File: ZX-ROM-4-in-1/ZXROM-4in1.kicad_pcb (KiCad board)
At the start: 2 copper layers, 27.9 x 35.6 mm, 9 parts, among them IC5 27C512, J1 Conn_01x14, J2 Conn_01x14, SW1 SW_DIP_x02

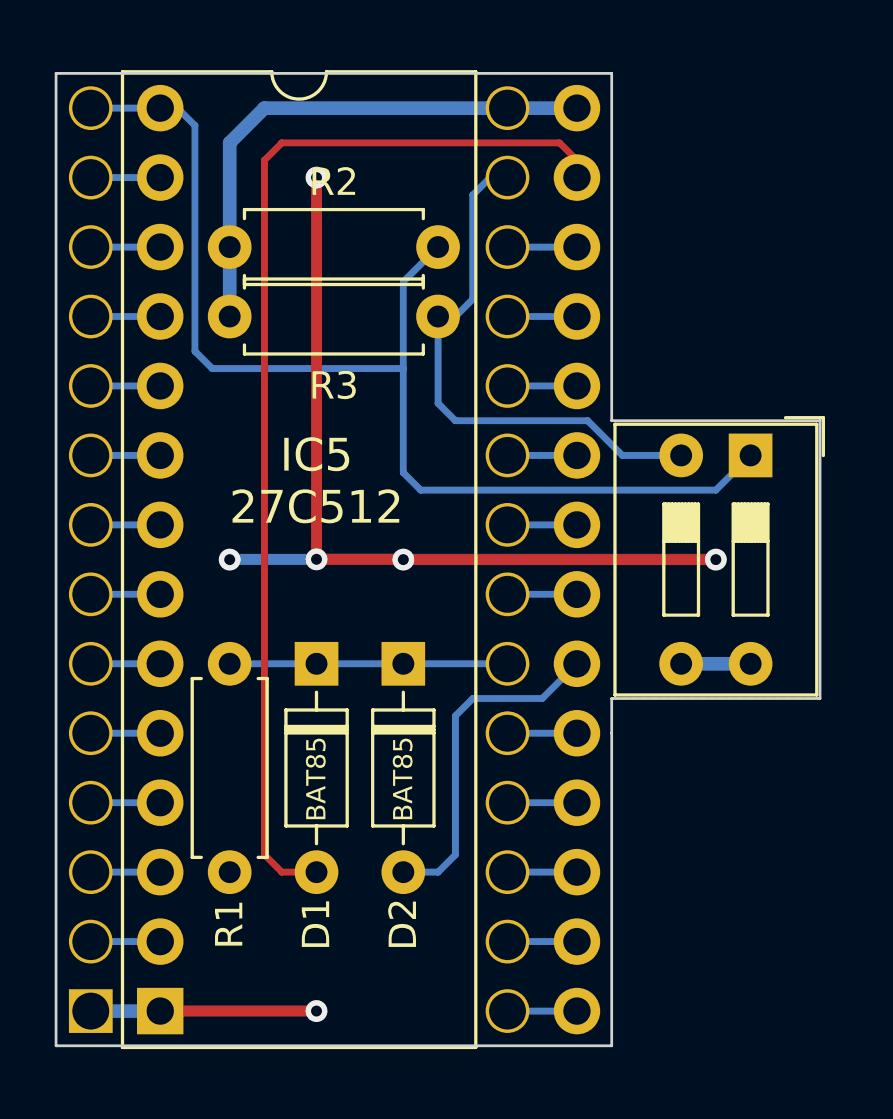
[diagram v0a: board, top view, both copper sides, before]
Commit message: New images, and adapter update
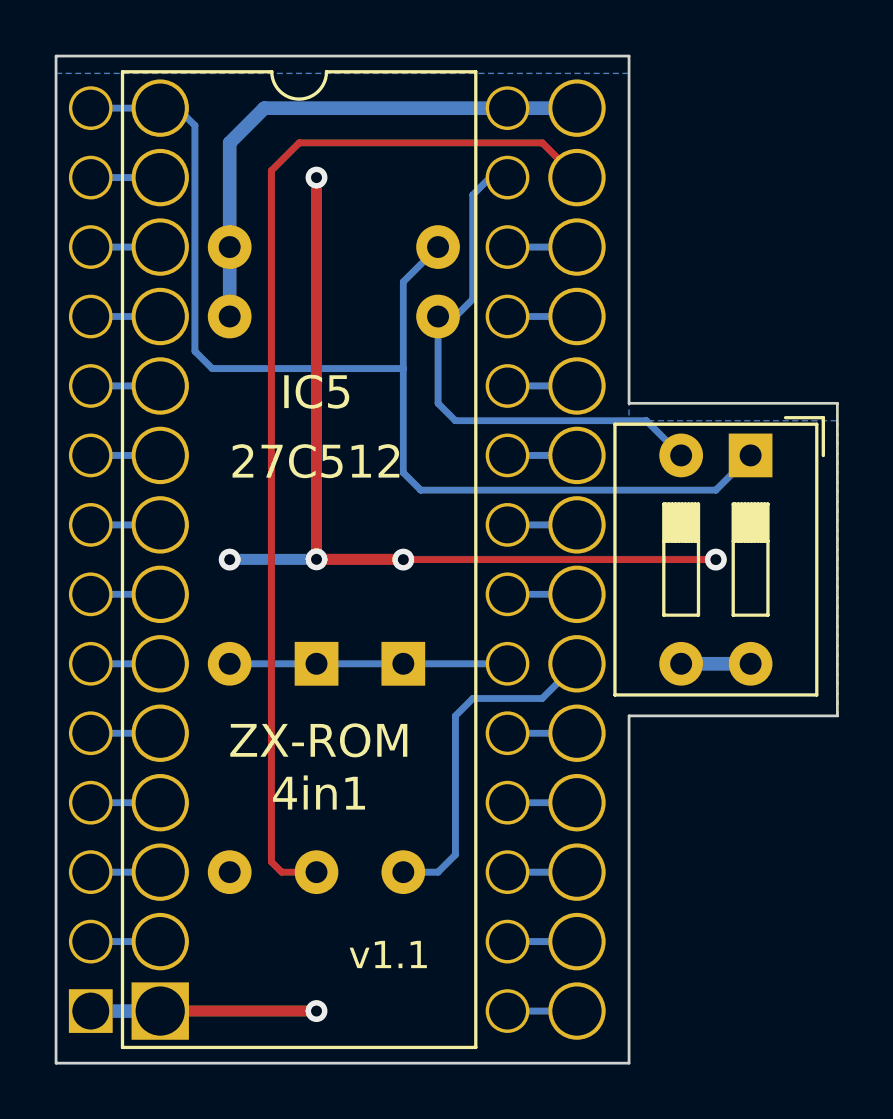
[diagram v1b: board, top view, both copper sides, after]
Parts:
- D1, D2, R1, R2, R3: moved to B.Cu
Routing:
- net /~{ROM_CS}: track 40.8 -> 39.8 mm
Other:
- board size 27.9 x 35.6 mm -> 28.6 x 36.8 mm
- board text added: "ZX-ROM 4in1"
- board text added: "v1.1"
- board text removed: "ZX ROM 4-in-1 27C512 Adapter v1.0"
